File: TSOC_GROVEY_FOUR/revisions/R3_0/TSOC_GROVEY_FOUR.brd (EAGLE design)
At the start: 44.5 x 30.5 mm, 39 parts, among them J2 JTAG-ISSPMIN, J3 4P-2.0-90D, J4 4P-2.0-90D, J5 4P-2.0-90D, J6 4P-2.0-90D, U1 CY8C4XXX-28

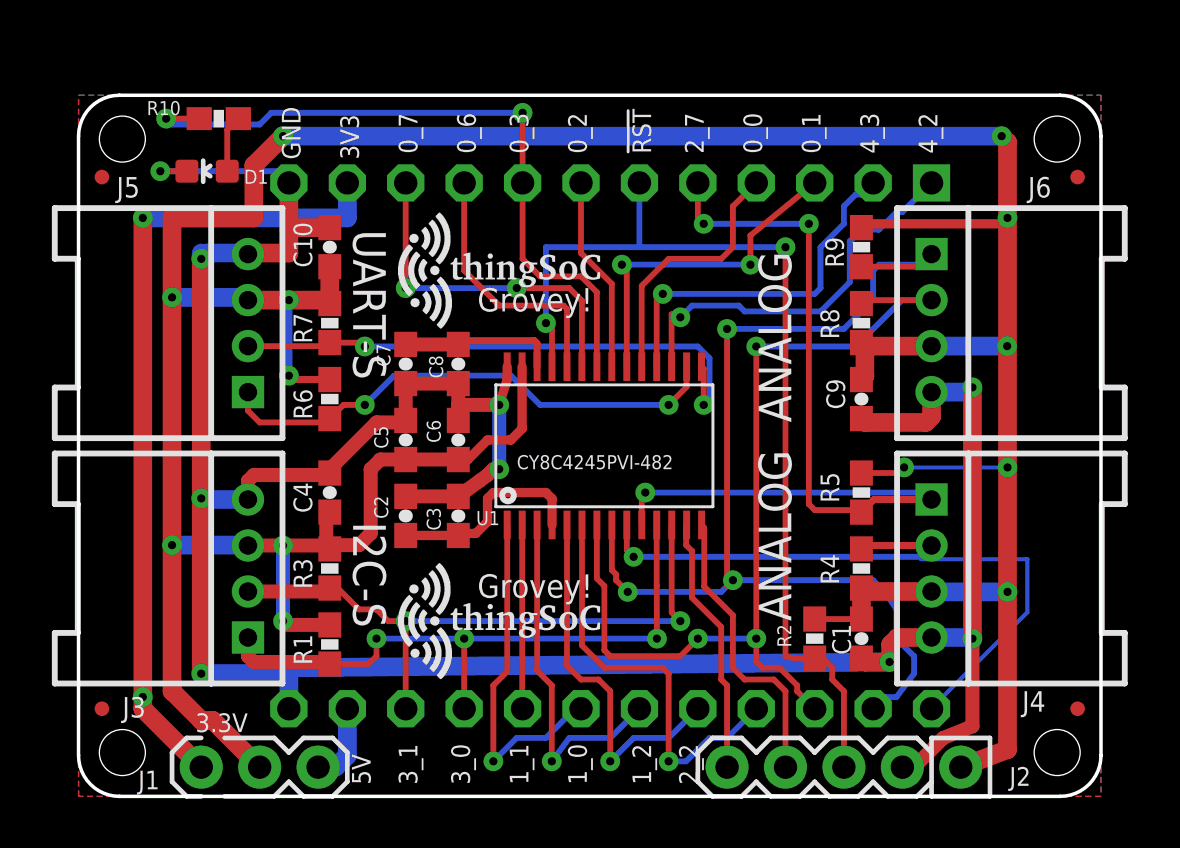
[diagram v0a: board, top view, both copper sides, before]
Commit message: add product images
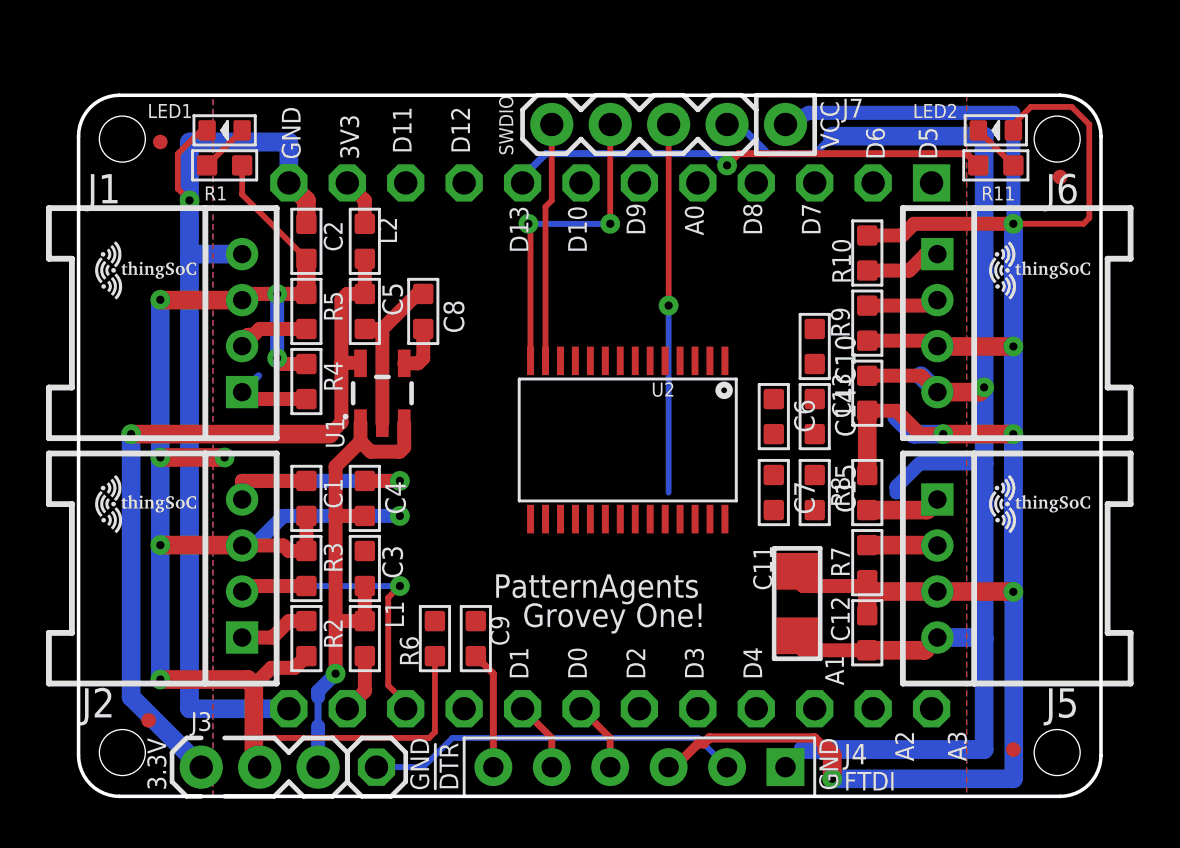
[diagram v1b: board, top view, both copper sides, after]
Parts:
- removed D1: (no value), TSOC-ESP8266-BASE:LED-0603
- removed U$4: TSOC-LOGO-MED, thingSoC:TSOC-LOGO-MED
- added $$U$2, $$U$3, U$103: TSOC-LOGO-SMALL, thingSoC:TSOC-LOGO-SML
- added C11: 22uF, TSOC_USBUART2:EIA-1206
- added C12, C13: 100nf, Seeed-Capacitor-2016:C0603
- added C14, C15: 1uF, Seeed-Capacitor-2016:C0603
- added GND: (no value), PatternAgents-ProtoPads:1X01
- added J7: JTAG-ISSPMIN, PatternAgents-Cypress:PSOC_JTAG_MINSILK
- added L1, L2: 120OHM-500MA, Seeed-Inductor-2016:L0603
- added LED1: GREEN-0603, Seeed-LED-2016:LED-0603
- added LED2: RED-0603, Seeed-LED-2016:LED-0603
- added R11: 1K 1/10W, Seeed-Resistor-2016:R0603
- added TSOC: TSOC-24-BB, thingSoC:TSOC-BB-S24
- added U2: CY8C4XXX-28, PatternAgents-Cypress:SSOP28
- C1, C10, C4, C9: value 1uF -> 100nf; device SparkFun-Passives:0603-CAP -> Seeed-Capacitor-2016:C0603
- C2: value 1uF -> 100nf; device PatternAgents-Misc:0603-CAP -> Seeed-Capacitor-2016:C0603
- C3: value 0.1uF -> 10uf; device PatternAgents-Misc:0603-CAP -> Seeed-Capacitor-2016:C0603
- C5: value 1uF -> 10uf; device PatternAgents-Misc:0603-CAP -> Seeed-Capacitor-2016:C0603
- C6: value 0.1uF -> 100nf; device PatternAgents-Misc:0603-CAP -> Seeed-Capacitor-2016:C0603
- C7: device PatternAgents-Misc:0603-CAP -> Seeed-Capacitor-2016:C0603
- C8: value 0.1uF -> 470Pf; device PatternAgents-Misc:0603-CAP -> Seeed-Capacitor-2016:C0603
- J1: value (none) -> 4P-2.0-90D; device PatternAgents-ProtoPads:JMP-3-NO-PTH-2.54 -> Seeed-Connector -2016:HW4-2.0-90D
- J2: value JTAG-ISSPMIN -> 4P-2.0-90D; device PatternAgents-Cypress:PSOC_JTAG_MINSILK -> Seeed-Connector -2016:HW4-2.0-90D
- J3: value 4P-2.0-90D -> NO; device Seeed-Connector -2016:HW4-2.0-90D -> PatternAgents-ProtoPads:JMP-3-NO-PTH-2.54
- J4: value 4P-2.0-90D -> 6p-2.54; device Seeed-Connector -2016:HW4-2.0-90D -> Seeed-Connector -2016:H6-2.54
- R1: value 2k2 -> 1K 1/10W; device SparkFun-Passives:0603-RES -> Seeed-Resistor-2016:R0603
- R10: value 1K -> 2.2K; device PatternAgents-Misc:0603-RES -> Seeed-Resistor-2016:R0603
- R2: value 10K -> 2.2K; device PatternAgents-Misc:0603-RES -> Seeed-Resistor-2016:R0603
- R3, R4, R5, R8, R9: value 2k2 -> 2.2K; device SparkFun-Passives:0603-RES -> Seeed-Resistor-2016:R0603
- R6: value DNP -> 10K 1/10W; device SparkFun-Passives:0603-RES -> Seeed-Resistor-2016:R0603
- R7: value DNP -> 2.2K; device SparkFun-Passives:0603-RES -> Seeed-Resistor-2016:R0603
- U$1: value TSOC-LOGO-MED -> TSOC-LOGO-SMALL; device thingSoC:TSOC-LOGO-MED -> thingSoC:TSOC-LOGO-SML
- U$101: value TSOC-LOGO-LRG -> TSOC-LOGO-SMALL; device thingSoC:TSOC-LOGO-LRG -> thingSoC:TSOC-LOGO-SML
- U$102: value TSOC-LOGO-SMALL -> TSOC-LOGO-LRG; device thingSoC:TSOC-LOGO-SML -> thingSoC:TSOC-LOGO-LRG
- U$3: value TSOC-24-BB -> TSOC-LOGO-SMALL; device thingSoC:TSOC-BB-S24 -> thingSoC:TSOC-LOGO-SML
- U1: value CY8C4XXX-28 -> MIC5219 3.3V; device PatternAgents-Cypress:SSOP28 -> TSOC-ESP8266-BASE:SOT23-5
- moved FID2 46.9 mm to (3.56, 28.4)
- moved FID3 41.7 mm to (42.7, 26.9)
- moved U$100 39.6 mm to (4.32, 15.2)
- moved J5 31.8 mm to (37.3, 9.91), turned to 270 degrees
- moved R10 28.8 mm to (34.3, 23.6)
- moved J2 27.6 mm to (7.11, 9.91), turned to 90 degrees
- moved U$101 26.2 mm to (7.37, 28.2)
- moved R7 25.6 mm to (34.3, 10.2), turned to 0 degrees
- moved R4 25.5 mm to (9.91, 18.0), turned to 180 degrees
- moved R5 25.4 mm to (9.91, 21.1), turned to 180 degrees
- moved U$102 25.3 mm to (31.0, 19.3)
- moved U$3 25.3 mm to (1.52, 22.9), turned to 0 degrees
- moved FID4 25.0 mm to (40.6, 2.03)
- moved C1 24.9 mm to (9.91, 13.0), turned to 180 degrees
- moved R2 22.1 mm to (9.91, 6.86), turned to 0 degrees
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- renumbered U$2 to $$U$1
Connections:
- new net !URST: C9.1, J4.6
- new net $1: TSOC.3B, TSOC.4B
- new net BYPASS1: C8.1, U1.4
- new net LEDR: LED2.-, R11.1
- new net TSOC_3V3: L2.2, TSOC.11B
- new net TSOC_5V0: L1.2, TSOC.11C
- net !XRES: now also C9.2, J7.3, R6.1, U2.25; no longer J2.3, R2.1, U$3.6B, U1.25
- net 3V3: now also C5.2, J3.1, L2.1, U1.5; no longer J1.1, U$3.11B
- net 5V0: now also C3.2, C4.1, J3.3, L1.1, U1.1, U1.3; no longer J1.3, U$3.11C
- net GND: now also C10.1, C11.2, C12.2, C13.2, C14.1, C15.1, C3.1, C5.1, C6.1, C7.1, GND.1, J1.4, J2.4, J4.1, J4.2, J7.2, LED1.-, TSOC.12B, TSOC.12C, U1.2, U2.28; no longer C10.2, C3.2, C5.2, C6.2, C7.2, C9.2, D1.C, J2.2, J3.4, J4.4, U$3.12B, U$3.12C, U1.28
- net N$17: now also LED1.+, R1.1; no longer D1.A, R10.1
- net P0_0: now also TSOC.6C, U2.19; no longer U$3.4B, U1.19
- net P0_1: now also TSOC.5C, U2.20; no longer U$3.3B, U1.20
- net P0_2: now also J5.2, R7.1, TSOC.4C, U2.21; no longer U$3.7B, U1.21
- net P0_3: now also J1.1, R11.2, R4.1, TSOC.3C, U2.22; no longer R10.2, U$3.8B, U1.22
- net P0_6: now also TSOC.1C, U2.24; no longer U$3.9B, U1.24
- net P0_7: now also J1.2, R5.1, TSOC.2C, U2.23; no longer U$3.10B, U1.23
- net P1_0: now also TSOC.1B, U2.1; no longer U$3.7C, U1.1
- net P1_1: now also TSOC.2B, U2.2; no longer U$3.8C, U1.2
- net P1_2: now also U2.3; no longer U$3.6C, U1.3
- net P1_7: now also C15.2, C6.2, U2.4; no longer C2.1, C3.1, U1.4
- net P2_2: now also TSOC.5B, U2.5; no longer U$3.5C, U1.5
- net P2_3: now also TSOC.6B, U2.6; no longer U$3.4C, U1.6
- net P2_4: now also J5.1, TSOC.7B, U2.7; no longer J6.2, U$3.3C, U1.7
- net P2_5: now also TSOC.8B, U2.8; no longer J6.1, R9.1, U$3.2C, U1.8
- net P2_6: now also J6.1, R10.1, TSOC.9B, U2.9; no longer J4.2, R4.1, U$3.1C, U1.9
- net P2_7: now also TSOC.10B, U2.10; no longer J4.1, R5.1, U$3.5B, U1.10
- net P3_0: now also J2.1, R2.1, TSOC.9C, U2.11; no longer J3.1, R1.1, U$3.9C, U1.11
- net P3_1: now also J2.2, TSOC.10C, U2.12; no longer J3.2, U$3.10C, U1.12
- net P3_2: now also J7.5, U2.13; no longer J2.5, U1.13
- net P3_3: now also J7.4, U2.14; no longer J2.4, U1.14
- net P4_0: now also J4.4, TSOC.7C, U2.15; no longer J5.2, R7.1, U1.15
- net P4_1: now also J4.5, TSOC.8C, U2.16; no longer J5.1, R6.1, U1.16
- net P4_2: now also J6.2, R9.1, U2.17; no longer U$3.1B, U1.17
- net P4_3: now also U2.18; no longer U$3.2B, U1.18
- net VCC: now also C10.2, C11.1, C12.1, C13.1, C14.2, C2.1, J1.3, J2.3, J3.2, J7.1, LED2.+, R10.2, U2.27; no longer C10.1, C4.1, C5.1, C6.1, C9.1, J1.2, J2.1, J3.3, U1.27
- net VCCD: now also C7.2, U2.26; no longer C7.1, C8.1, U1.26
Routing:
- net P2_5: track 47.2 -> 0.00 mm, vias 3 -> 0
- net P2_7: track 38.4 -> 0.00 mm, vias 3 -> 0
- net P2_4: track 41.4 -> 3.24 mm, vias 3 -> 0
- net !XRES: track 43.4 -> 16.0 mm, vias 2 -> 1
- net P2_6: track 30.7 -> 3.34 mm, vias 1 -> 0
- net P3_0: track 27.6 -> 3.12 mm, vias 3 -> 0
- net GND: track 125.6 -> 147.6 mm, vias 9 -> 3
- net P4_0: track 24.2 -> 3.07 mm, vias 2 -> 0
- net P4_1: track 22.7 -> 3.07 mm, vias 2 -> 0
- net 5V0: track 3.51 -> 23.0 mm, vias 0 -> 1
- net P2_3: track 18.1 -> 0.00 mm, vias 1 -> 0
- net P2_2: track 16.3 -> 0.00 mm, vias 1 -> 0
- net P4_3: track 16.0 -> 0.00 mm, vias 1 -> 0
- net P1_2: track 15.4 -> 0.00 mm, vias 1 -> 0
- net P1_0: track 15.3 -> 0.00 mm, vias 1 -> 0
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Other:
- board text added: "A0"
- board text added: "A1"
- board text added: "A2"
- board text added: "A3"
- board text added: "A4"
- board text added: "A5"
- board text added: "D0"
- board text added: "D1"
- board text added: "D10"
- board text added: "D11"
- board text added: "D12"
- board text added: "D13"
- board text added: "D2"
- board text added: "D3"
- board text added: "D4"
- board text added: "D5"
- board text added: "D6"
- board text added: "D7"
- board text added: "D8"
- board text added: "D9"
- board text added: "FTDI"
- board text added: "Grovey One!"
- board text added: "J1"
- board text added: "J3"
- board text added: "J4"
- board text added: "J5"
- board text added: "J6"
- board text added: "JTAG"
- board text added: "Rev. 3.0"
- board text added: "SWDIO"
- board text added: "TSOC_GROVEY_FOUR!"
- board text added: "UART"
- board text removed: "!CS"
- board text removed: "!DCD"
- board text removed: "!DSR"
- board text removed: "!IRQ"
- board text removed: "!RI"
- board text removed: "!RST"
- board text removed: "!RTS"
- board text removed: "0_0"
- board text removed: "0_1"
- board text removed: "0_2"
- board text removed: "0_3"
- board text removed: "0_6"
- board text removed: "0_7"
- board text removed: "1_0"
- board text removed: "1_1"
- board text removed: "1_2"
- board text removed: "2_2"
- board text removed: "2_3"
- board text removed: "2_4"
- board text removed: "2_5"
- board text removed: "2_6"
- board text removed: "2_7"
- board text removed: "3_0"
- board text removed: "3_1"
- board text removed: "4_2"
- board text removed: "4_3"
- board text removed: "5V"
- board text removed: "ANALOG"
- board text removed: "CY8C4245PVI-482"
- board text removed: "Grovey!"
- board text removed: "I2C-S"
- board text removed: "IO1"
- board text removed: "IO2"
- board text removed: "MISO"
- board text removed: "MOSI"
- board text removed: "P2_4"
- board text removed: "P2_5"
- board text removed: "P2_6"
- board text removed: "P2_7"
- board text removed: "P3_0"
- board text removed: "P3_1"
- board text removed: "P4_0"
- board text removed: "P4_1"
- board text removed: "RXD"
- board text removed: "Rev. 2.0"
- board text removed: "SCK"
- board text removed: "SCL"
- board text removed: "SDA"
- board text removed: "SS1"
- board text removed: "SS2"
- board text removed: "TXD"
- board text removed: "UART-S"
